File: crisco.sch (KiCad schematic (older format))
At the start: 45 parts, among them J1 LED, J2 OLED, U1 ProMicro

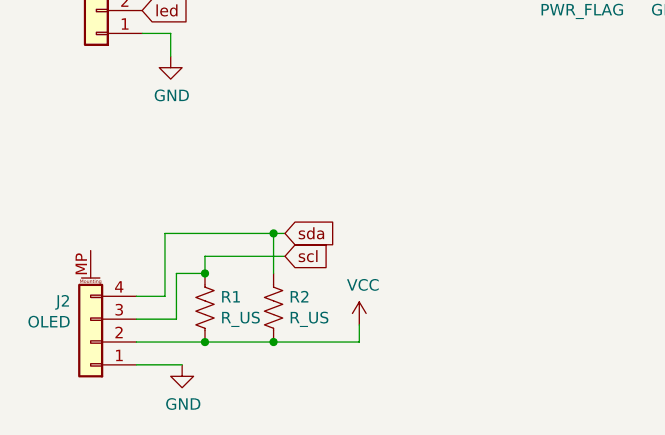
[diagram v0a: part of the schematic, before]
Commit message: update gerber
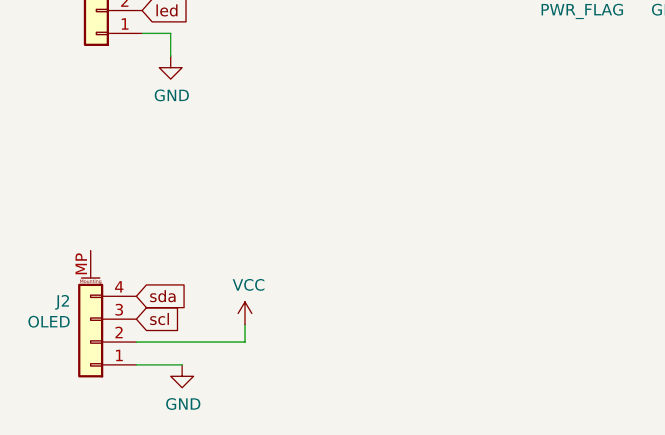
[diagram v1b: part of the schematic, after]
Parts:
- removed R1, R2: R_US, Resistor_THT:R_Axial_DIN0204_L3.6mm_D1.6mm_P5.08mm_Horizontal, symbol Device:R_US
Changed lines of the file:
@@
 L power:VCC #PWR0109
 U 1 1 61CCE8B0
-P 3125 5175
-F 0 "#PWR0109" H 3125 5025 50  0001 C CNN
-F 1 "VCC" H 3142 5348 50  0000 C CNN
-F 2 "" H 3125 5175 50  0001 C CNN
-F 3 "" H 3125 5175 50  0001 C CNN
-	1    3125 5175
+P 2625 5175
+F 0 "#PWR0109" H 2625 5025 50  0001 C CNN
+F 1 "VCC" H 2642 5348 50  0000 C CNN
+F 2 "" H 2625 5175 50  0001 C CNN
+F 3 "" H 2625 5175 50  0001 C CNN
+	1    2625 5175
 	1    0    0    -1
 $EndComp
@@
 	1    0    0    -1
 $EndComp
-Text GLabel 2800 4875 2    50   Input ~ 0
+Text GLabel 2150 5150 2    50   Input ~ 0
 scl
-Text GLabel 2800 4775 2    50   Input ~ 0
+Text GLabel 2150 5050 2    50   Input ~ 0
 sda
 Wire Wire Line
-	3125 5250 3125 5175
+	2625 5250 2625 5175
 Wire Wire Line
 	2150 5350 2350 5350
 NoConn ~ 3650 2200
-$Comp
-L Device:R_US R1
-U 1 1 61D4AEF9
-P 2450 5100
-F 0 "R1" H 2518 5146 50  0000 L CNN
-F 1 "R_US" H 2518 5055 50  0000 L CNN
-F 2 "Resistor_THT:R_Axial_DIN0204_L3.6mm_D1.6mm_P5.08mm_Horizontal" V 2490 5090 50  0001 C CNN
-F 3 "~" H 2450 5100 50  0001 C CNN
-	1    2450 5100
-	1    0    0    -1
-$EndComp
-$Comp
-L Device:R_US R2
-U 1 1 61D4BA80
-P 2750 5100
-F 0 "R2" H 2818 5146 50  0000 L CNN
-F 1 "R_US" H 2818 5055 50  0000 L CNN
-F 2 "Resistor_THT:R_Axial_DIN0204_L3.6mm_D1.6mm_P5.08mm_Horizontal" V 2790 5090 50  0001 C CNN
-F 3 "~" H 2750 5100 50  0001 C CNN
-	1    2750 5100
-	1    0    0    -1
-$EndComp
 Wire Wire Line
-	2750 5250 3125 5250
-Wire Wire Line
-	2750 5250 2450 5250
-Connection ~ 2750 5250
-Wire Wire Line
-	2450 5250 2150 5250
-Connection ~ 2450 5250
-Wire Wire Line
-	2325 5150 2150 5150
-Wire Wire Line
-	2275 5050 2275 4775
-Wire Wire Line
-	2275 4775 2750 4775
-Wire Wire Line
-	2325 4950 2450 4950
-Wire Wire Line
-	2450 4950 2450 4875
-Wire Wire Line
-	2450 4875 2800 4875
-Wire Wire Line
-	2325 4950 2325 5150
-Connection ~ 2450 4950
-Wire Wire Line
-	2750 4775 2750 4950
-Connection ~ 2750 4775
-Wire Wire Line
-	2750 4775 2800 4775
-Wire Wire Line
-	2150 5050 2275 5050
+	2150 5250 2625 5250
 $EndSCHEMATC
